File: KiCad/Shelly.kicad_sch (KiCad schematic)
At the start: 26 parts, among them J1 Shelly 1, J2 Other, J3 USB-C, Q1 PMF170XP,115, Q2 PMF250XNEX, U1 FT231XQ, U2 LMR16006+FB

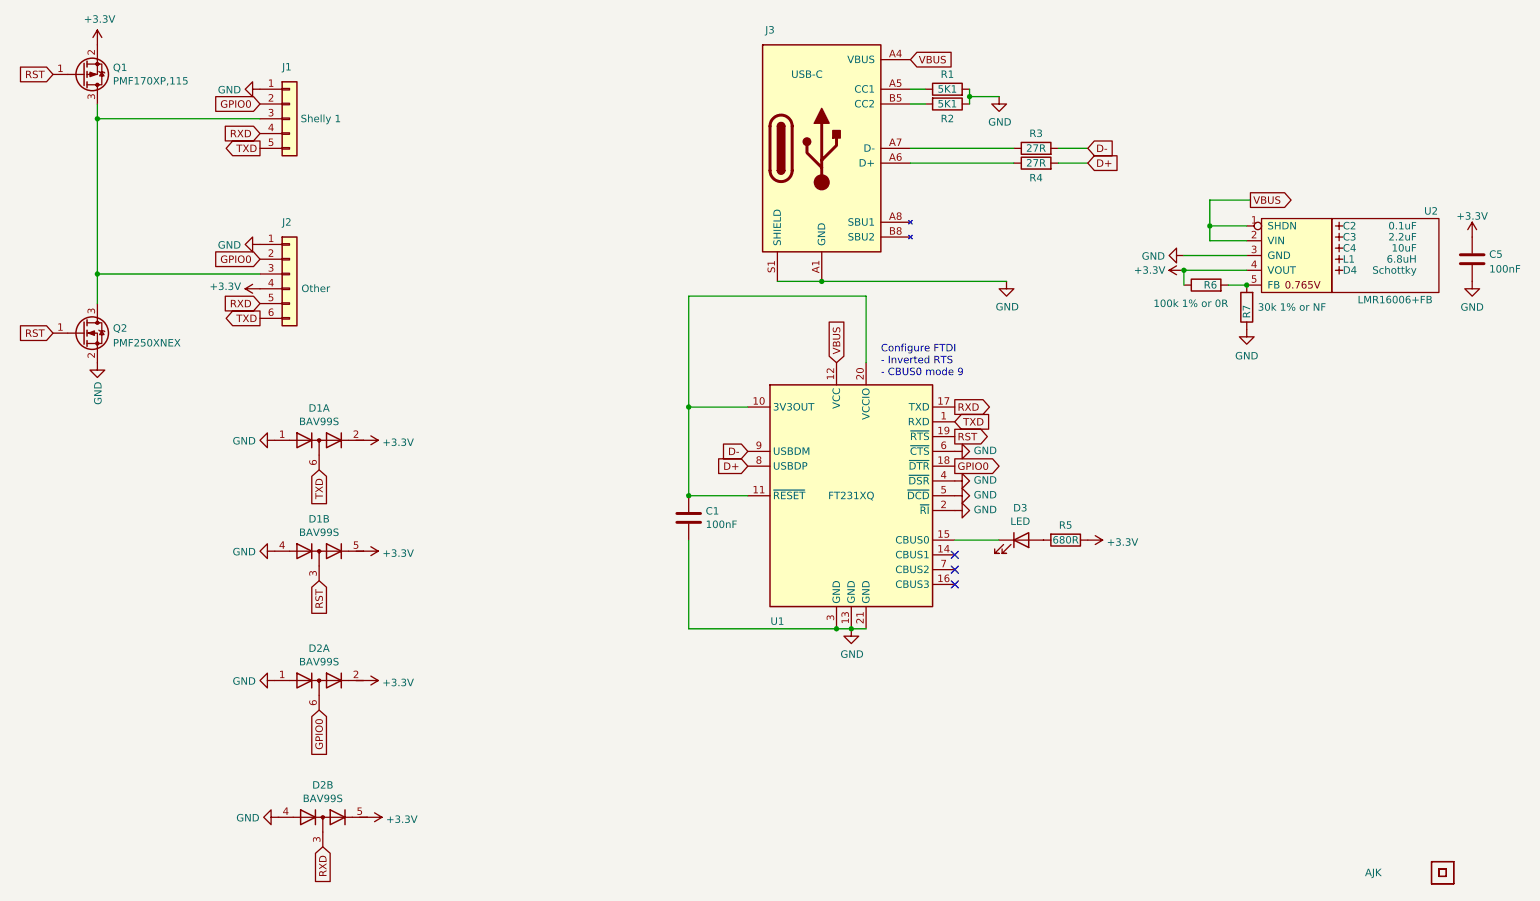
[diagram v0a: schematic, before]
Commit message: Library update
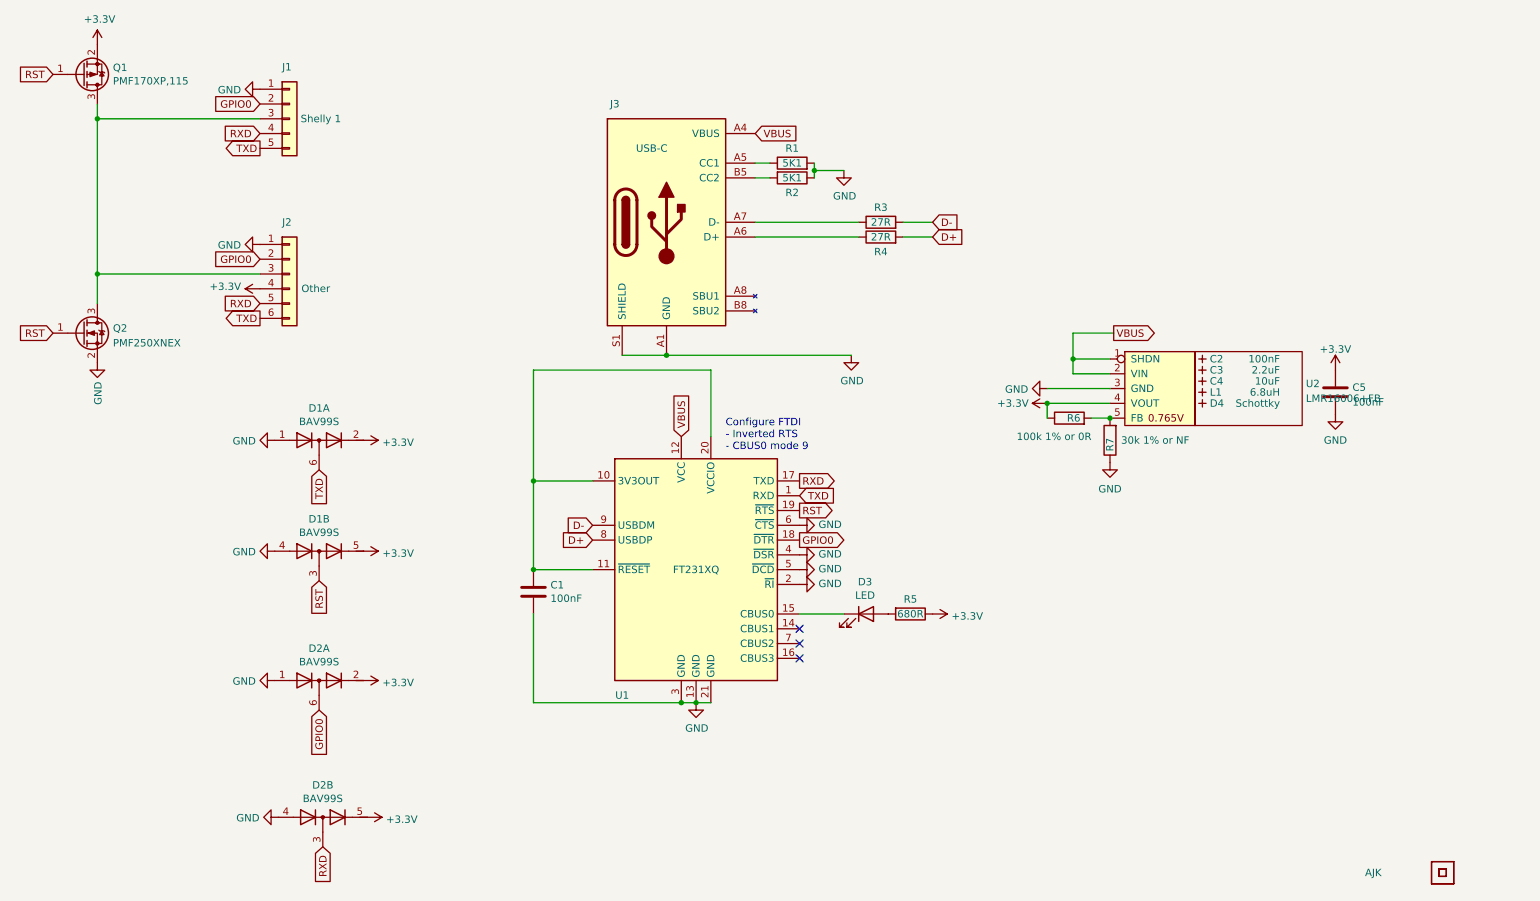
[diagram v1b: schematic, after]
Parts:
- C2: value 0.1uF -> 100nF; footprint RevK:Hidden -> RevK:C_0603_
- C3, C4: footprint RevK:Hidden -> RevK:C_0805_
- D4: footprint RevK:Hidden -> RevK:D_1206_
- L1: footprint RevK:Hidden -> RevK:L_4x4_
- U2: footprint RevK:RegulatorBlockFB -> RevK:SOT-23-Thin-6-Reg
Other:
- moved on the sheet: C1, C5, D3, J3, R1, R2, R3, R4, R5, R6, R7, U1
